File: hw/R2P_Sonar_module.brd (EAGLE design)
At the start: 40 x 40 mm, 36 parts, among them U1 STM32F103CX, U5 LD3985XX, X1 MICROMATCH-4, X2 MICROMATCH-6, X3 MICROMATCH-6-SIDE

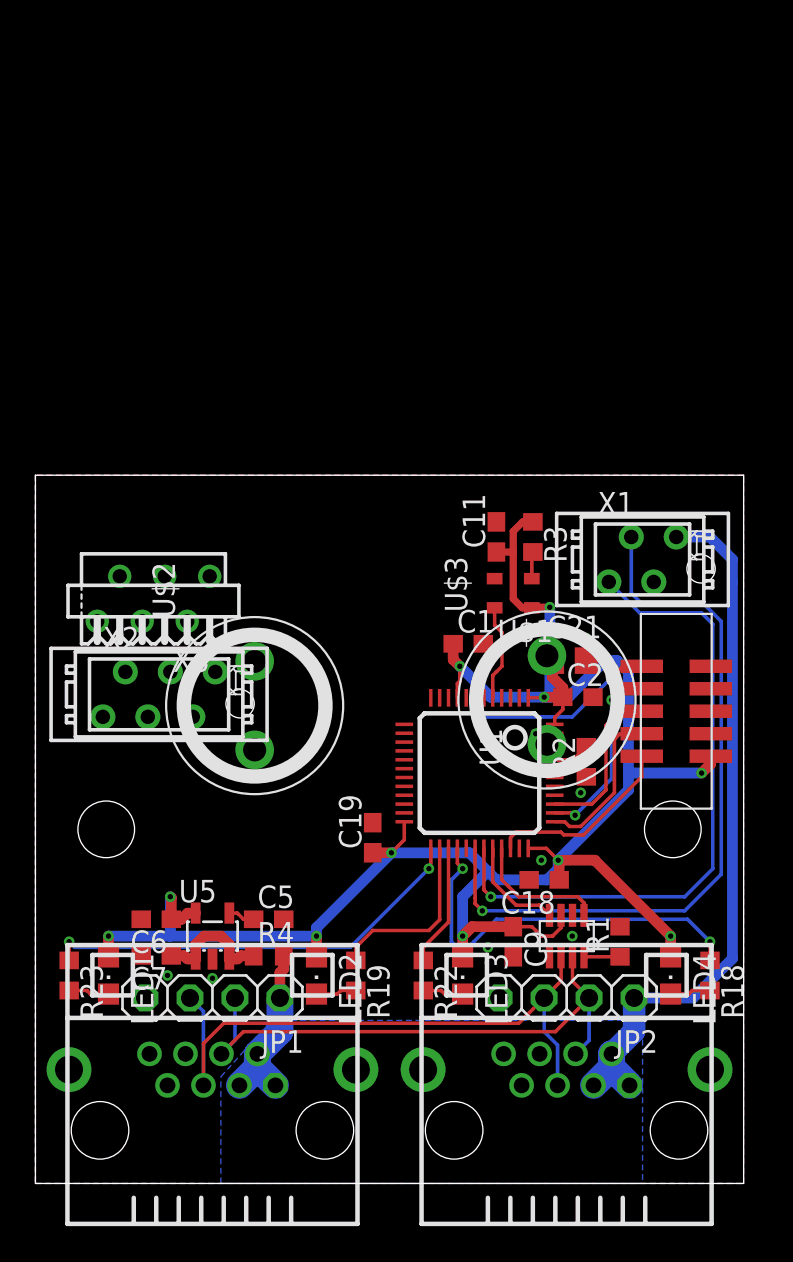
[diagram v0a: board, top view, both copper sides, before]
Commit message: Ongoing layout
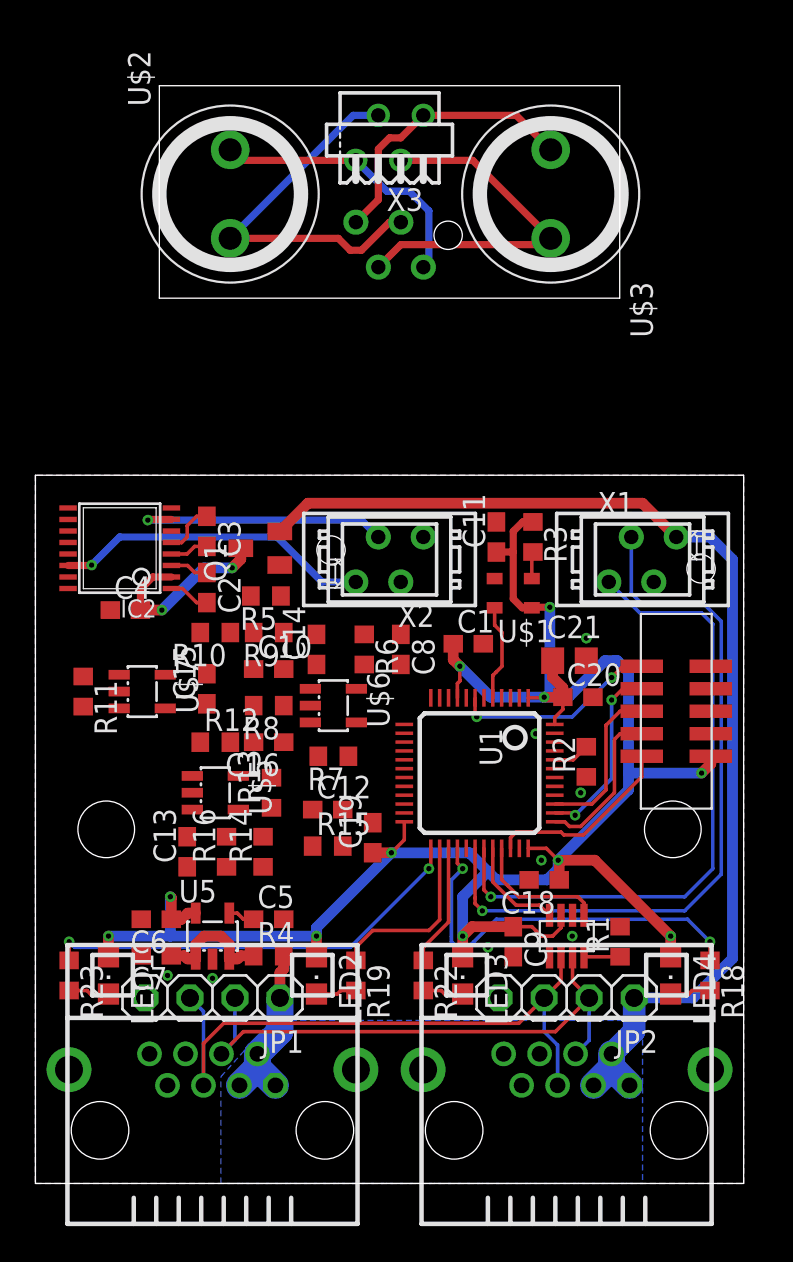
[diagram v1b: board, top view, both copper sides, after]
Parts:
- added C10, C12, C13, C14, C15, C16, C2, C3, C4, C8: 100n, rcl:C0603
- added IC2: MAX3232CUE, maxim:TSSOP16
- added Q1: BC807-16SMD, transistor-pnp:SOT23-BEC
- added R10, R11, R12, R13, R14, R15, R16, R6, R8, R9: 2k2, rcl:R0603
- added R5, R7: 10k, rcl:R0603
- added U$5: LMV331, texas-instruments:SOT23-5L
- added U$6, U$7: TS461, st:SOT23-5L
- added X4: MICROMATCH-4, tyco:MICROMATCH-4
- X2: value MICROMATCH-6 -> MICROMATCH-4; device tyco:MICROMATCH-6 -> tyco:MICROMATCH-4
- X3: value MICROMATCH-6-SIDE -> MICROMATCH-4-SIDE; device tyco:MICROMATCH-6-SIDE -> apbteam_con-amp-micromatch:MICROMATCH-4-SIDE
- moved X3 29.3 mm to (20.0, 59.1)
- moved U$2 28.9 mm to (11.0, 55.9)
- moved U$3 28.6 mm to (29.1, 55.9), turned to 270 degrees
- moved X2 15.1 mm to (20.0, 35.2), turned to 180 degrees
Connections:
- new net N$10: C4.2, IC2.2, Q1.C
- new net N$11: C8.2, R6.1
- new net N$12: U$2.P$1, X3.1, X4.1
- new net N$13: U$2.P$2, X3.2, X4.2
- new net N$14: U$3.P$1, X3.3, X4.3
- new net N$16: U$3.P$2, X3.4, X4.4
- new net N$17: Q1.B, R5.1
- new net N$19: R5.2
- new net N$21: R6.2, R7.1, U$6.4
- new net N$23: R7.2, R8.1, U$6.1
- new net N$24: C10.1, R8.2
- new net N$25: C10.2, R9.1
- new net N$26: R10.1, R9.2, U$7.4
- new net N$27: R10.2, R11.1, U$7.1
- new net N$28: R11.2, R12.1, U$5.1
- new net N$30: C13.2, R16.2, U$5.3
- new net N$6: C2.2, IC2.1
- new net N$7: C2.1, IC2.3
- new net N$8: C3.2, IC2.4
- new net N$9: C3.1, IC2.5
- new net RX1: R12.2, R13.1, U$5.4
- new net TX1: IC2.11
- new net TX2: IC2.10
- new net URX1: C8.1, X2.3
- new net UTX1: IC2.14, X2.1
- new net UTX2: IC2.7, X2.2
- new net VCC: IC2.16
- new net VREF: C12.2, R14.1, R15.2, R16.1, U$6.3, U$7.3
- net +5V: now also C14.2, C15.2, C16.2, Q1.E, R13.2, R14.2, U$5.5, U$6.5, U$7.5
- net GND: now also C12.1, C13.1, C14.1, C15.1, C16.1, C4.1, IC2.13, IC2.15, IC2.6, IC2.8, R15.1, U$5.2, U$6.2, U$7.2, X2.4
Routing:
- net +5V: track 51.4 -> 73.7 mm
- net N$13: track 0.00 -> 21.8 mm
- net N$14: track 0.00 -> 20.7 mm
- net UTX1: track 0.00 -> 18.0 mm, vias 0 -> 1
- net N$16: track 0.00 -> 16.0 mm
- net N$12: track 0.00 -> 16.0 mm
- net UTX2: track 0.00 -> 14.8 mm, vias 0 -> 1
- net N$10: track 0.00 -> 10.7 mm, vias 0 -> 2
- net N$9: track 0.00 -> 2.99 mm
- net N$6: track 0.00 -> 2.33 mm
- net N$8: track 0.00 -> 2.18 mm
- net N$7: track 0.00 -> 2.17 mm
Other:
- board size 40 x 40 mm -> 40 x 62 mm
